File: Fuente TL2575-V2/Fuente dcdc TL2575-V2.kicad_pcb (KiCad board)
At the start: 2 copper layers, 55.9 x 38.1 mm, 22 parts, among them U1 TL2575

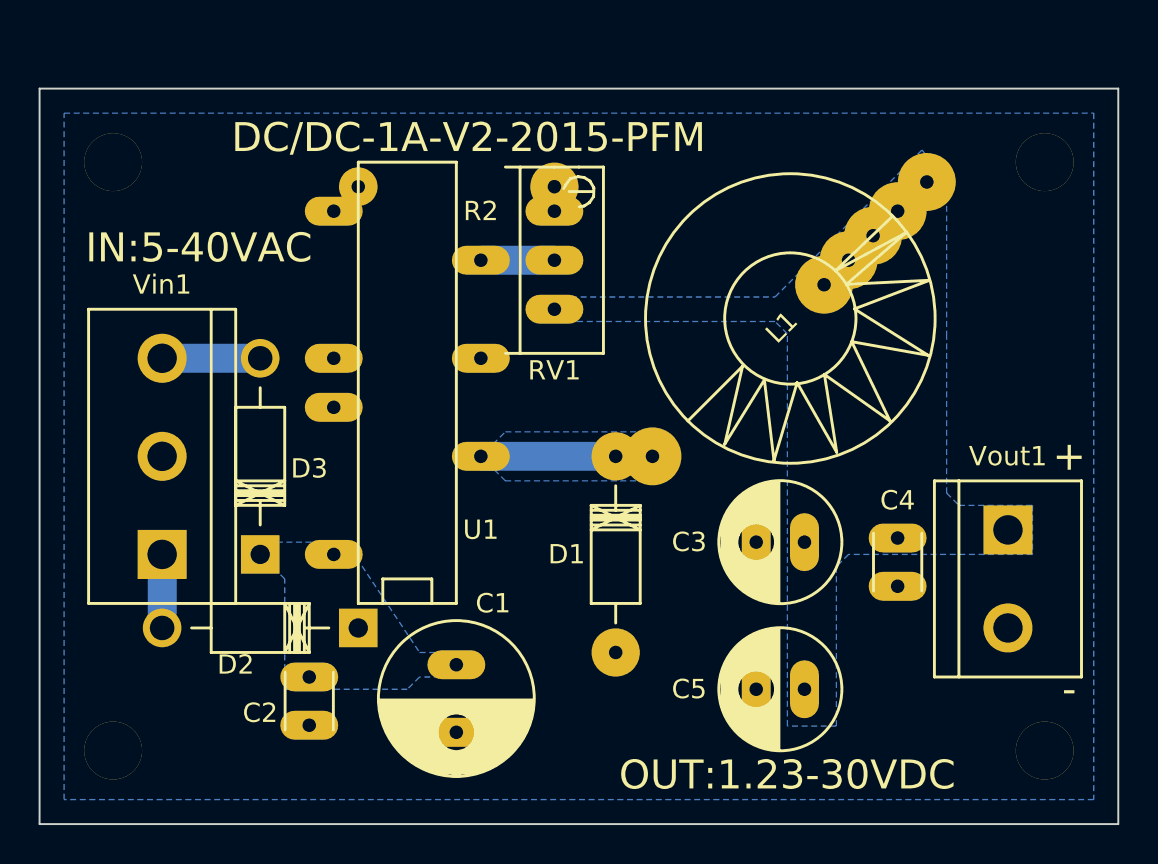
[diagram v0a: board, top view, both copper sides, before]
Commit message: Finalizando TL2575-V2
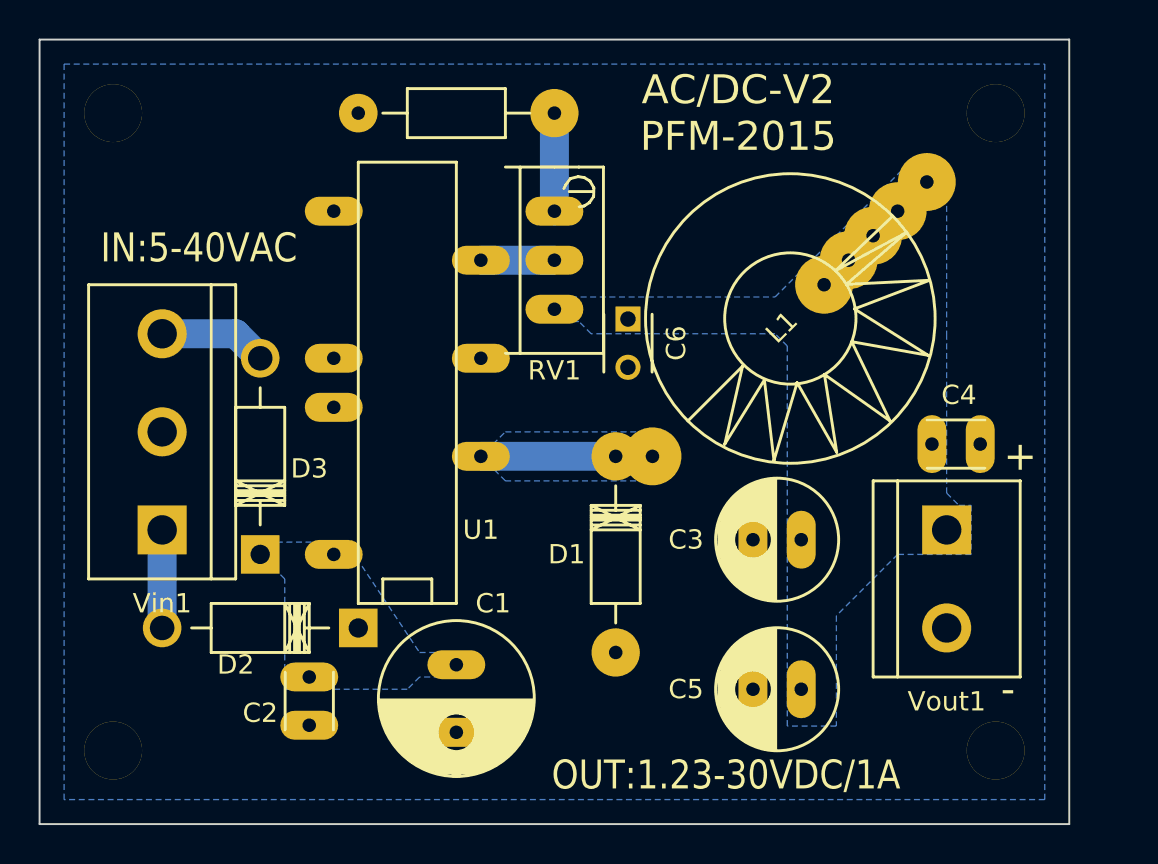
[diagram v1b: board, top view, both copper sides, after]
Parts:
- added C6: 100nF, Capacitors_ThroughHole:C_Disc_D3_P2.5, F.Cu at (128.3, 48.8)
- R2: moved to F.Cu
- Vin1: value CONN_01X03 -> VIN
- Vout1: value CONN_01X02 -> VOUT
- moved C4 5.18 mm to (144.0, 55.2), turned to 0 degrees
- moved R2 3.81 mm to (119.4, 38.1)
- moved REF** 3.59 mm to (147.3, 38.1)
- moved Vout1 3.18 mm to (144.8, 62.2)
- moved REF** 2.54 mm to (147.3, 71.1)
- moved REF** 2.54 mm to (101.6, 38.1)
- moved Vin1 1.27 mm to (104.1, 54.6)
- moved C3 0.21 mm to (137.2, 60.2)
- moved C5 0.17 mm to (137.2, 67.9)
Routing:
- net Net-(R2-Pad1): track 1.27 -> 5.08 mm
- net Net-(D2-Pad1): track 3.81 -> 5.08 mm
- net Net-(D3-Pad1): track 5.08 -> 5.61 mm
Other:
- board size 55.9 x 38.1 mm -> 53.3 x 40.6 mm
- board text added: "AC/DC-V2 PFM-2015"
- board text added: "OUT:1.23-30VDC/1A"
- board text removed: "DC/DC-1A-V2-2015-PFM"
- board text removed: "OUT:1.23-30VDC"
